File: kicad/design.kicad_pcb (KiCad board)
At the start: 2 copper layers, 20 x 15 mm, 1 part, among them U1 CH32L103K8U6

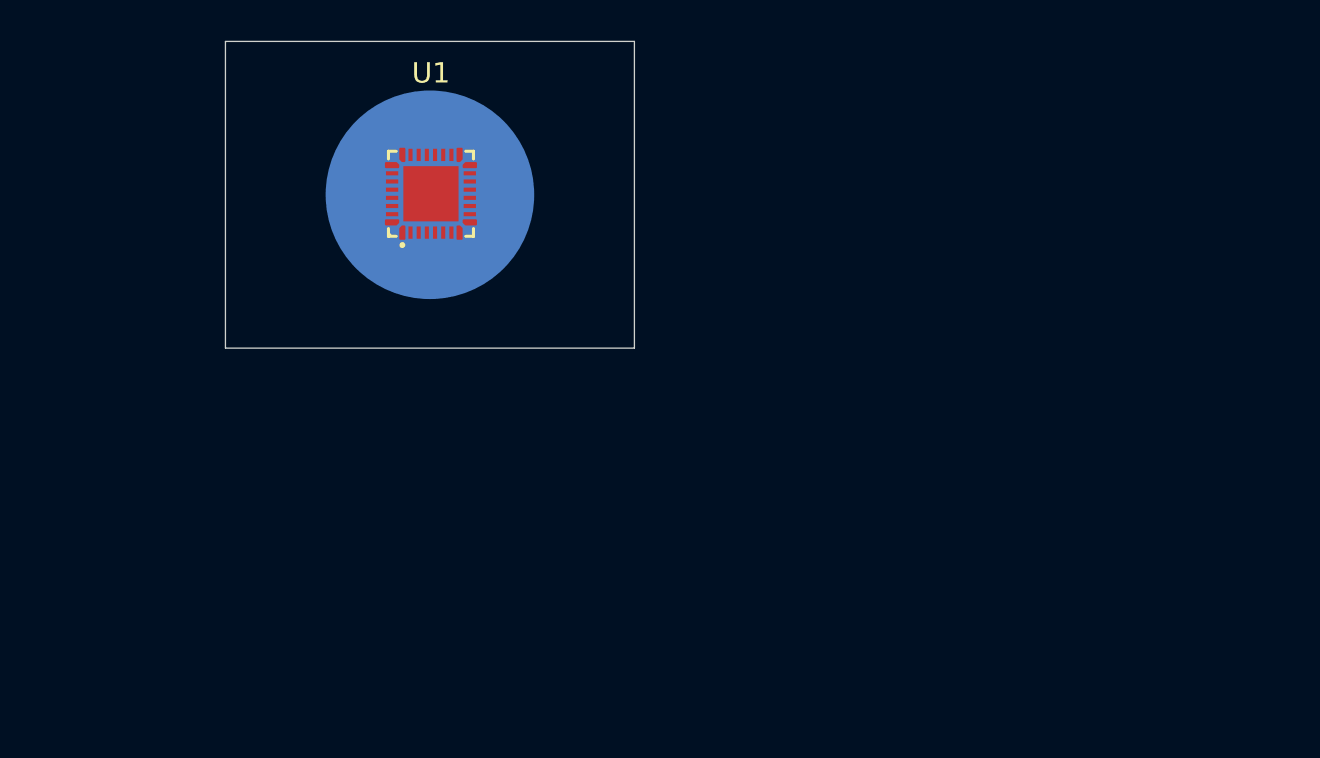
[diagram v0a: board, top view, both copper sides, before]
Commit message: I dont remember last commit idk
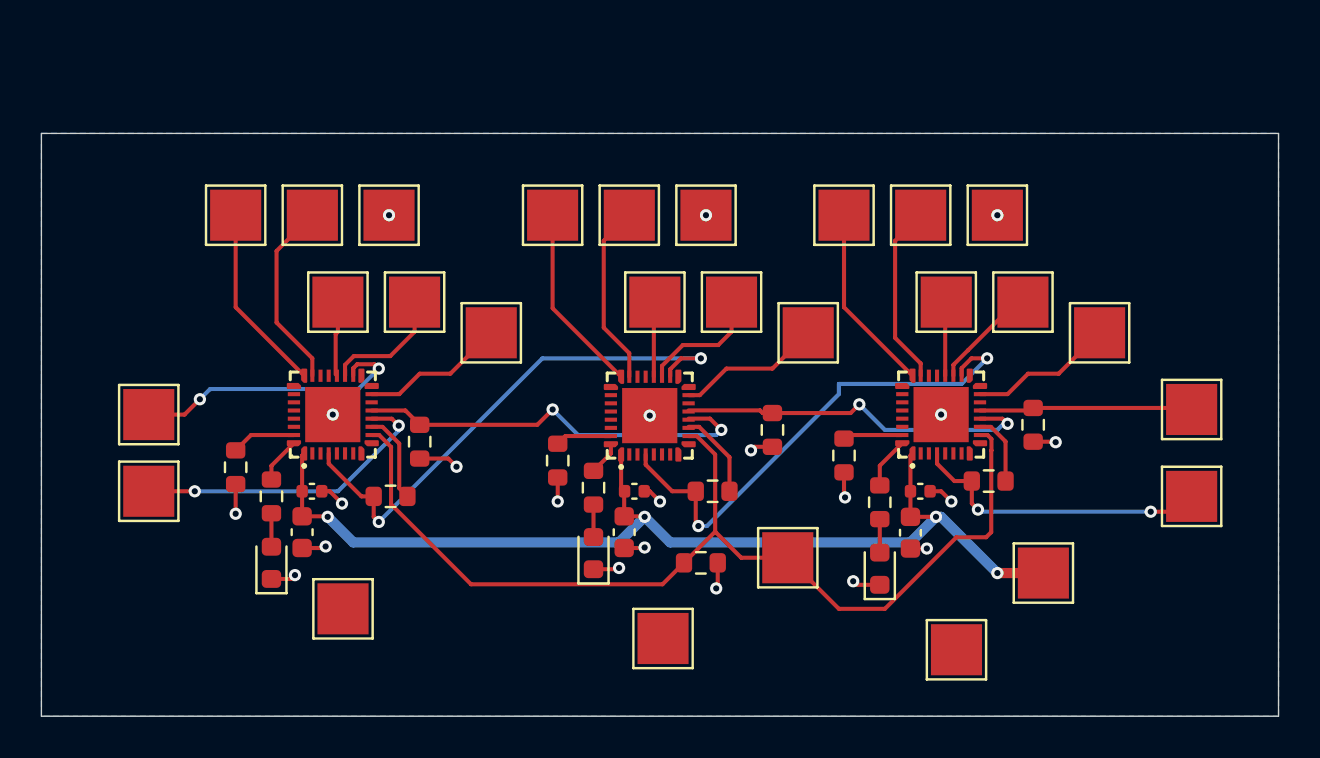
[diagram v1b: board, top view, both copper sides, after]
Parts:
- removed U1: CH32L103K8U6, LIB:QFN-32_L4.0-W4.0-P0.40-BL-EP2.7-A
- added C2: 4.7u, Capacitor_SMD:C_0603_1608Metric, F.Cu at (158.5, 89.0)
- added C3: 0.1u, Capacitor_SMD:C_0402_1005Metric, F.Cu at (159.0, 87.0)
- added C4: 0.1u, Capacitor_SMD:C_0402_1005Metric, F.Cu at (145.0, 87.0)
- added C5: 4.7u, Capacitor_SMD:C_0603_1608Metric, F.Cu at (144.5, 89.0)
- added C6: 0.1u, Capacitor_SMD:C_0402_1005Metric, F.Cu at (129.2, 87.0)
- added C7: 4.7u, Capacitor_SMD:C_0603_1608Metric, F.Cu at (128.8, 89.0)
- added D1: LED, LED_SMD:LED_0603_1608Metric, F.Cu at (157.0, 90.8)
- added D2: LED, LED_SMD:LED_0603_1608Metric, F.Cu at (143.0, 90.0)
- added D3: LED, LED_SMD:LED_0603_1608Metric, F.Cu at (127.2, 90.5)
- added R1: 0, Resistor_SMD:R_0603_1608Metric, F.Cu at (162.3, 86.5)
- added R10: 10k, Resistor_SMD:R_0603_1608Metric, F.Cu at (134.5, 84.6)
- added R11: 470, Resistor_SMD:R_0603_1608Metric, F.Cu at (157.0, 87.5)
- added R12: 470, Resistor_SMD:R_0603_1608Metric, F.Cu at (143.0, 86.8)
- added R13: 470, Resistor_SMD:R_0603_1608Metric, F.Cu at (127.2, 87.2)
- added R2: 4.7k, Resistor_SMD:R_0603_1608Metric, F.Cu at (155.2, 85.2)
- added R3: 4.7k, Resistor_SMD:R_0603_1608Metric, F.Cu at (141.2, 85.5)
- added R4: 4.7k, Resistor_SMD:R_0603_1608Metric, F.Cu at (125.5, 85.8)
- added R5: 10k, Resistor_SMD:R_0603_1608Metric, F.Cu at (148.2, 90.5)
- added R6: 0, Resistor_SMD:R_0603_1608Metric, F.Cu at (148.8, 87.0)
- added R7: 0, Resistor_SMD:R_0603_1608Metric, F.Cu at (133.1, 87.2)
- added R8: 10k, Resistor_SMD:R_0603_1608Metric, F.Cu at (164.5, 83.8)
- added R9: 10k, Resistor_SMD:R_0603_1608Metric, F.Cu at (151.8, 84.0)
- added TP1: TestPoint, TestPoint:TestPoint_Pad_2.5x2.5mm, F.Cu at (121.2, 83.2)
- added TP10: TestPoint, TestPoint:TestPoint_Pad_2.5x2.5mm, F.Cu at (125.5, 73.5)
- added TP11: TestPoint, TestPoint:TestPoint_Pad_2.5x2.5mm, F.Cu at (162.8, 73.5)
- added TP12: TestPoint, TestPoint:TestPoint_Pad_2.5x2.5mm, F.Cu at (148.5, 73.5)
- added TP13: TestPoint, TestPoint:TestPoint_Pad_2.5x2.5mm, F.Cu at (133.0, 73.5)
- added TP14: TestPoint, TestPoint:TestPoint_Pad_2.5x2.5mm, F.Cu at (165.0, 91.0)
- added TP15: TestPoint, TestPoint:TestPoint_Pad_2.5x2.5mm, F.Cu at (152.5, 90.2)
- added TP16: TestPoint, TestPoint:TestPoint_Pad_2.5x2.5mm, F.Cu at (167.8, 79.2)
- added TP17: TestPoint, TestPoint:TestPoint_Pad_2.5x2.5mm, F.Cu at (153.5, 79.2)
- added TP18: TestPoint, TestPoint:TestPoint_Pad_2.5x2.5mm, F.Cu at (138.0, 79.2)
- added TP19: TestPoint, TestPoint:TestPoint_Pad_2.5x2.5mm, F.Cu at (164.0, 77.8)
- added TP2: TestPoint, TestPoint:TestPoint_Pad_2.5x2.5mm, F.Cu at (172.2, 87.2)
- added TP20: TestPoint, TestPoint:TestPoint_Pad_2.5x2.5mm, F.Cu at (149.8, 77.8)
- added TP21: TestPoint, TestPoint:TestPoint_Pad_2.5x2.5mm, F.Cu at (134.2, 77.8)
- added TP22: TestPoint, TestPoint:TestPoint_Pad_2.5x2.5mm, F.Cu at (160.2, 77.8)
- added TP23: TestPoint, TestPoint:TestPoint_Pad_2.5x2.5mm, F.Cu at (146.0, 77.8)
- added TP24: TestPoint, TestPoint:TestPoint_Pad_2.5x2.5mm, F.Cu at (130.5, 77.8)
- added TP25: TestPoint, TestPoint:TestPoint_Pad_2.5x2.5mm, F.Cu at (160.8, 94.8)
- added TP26: TestPoint, TestPoint:TestPoint_Pad_2.5x2.5mm, F.Cu at (146.4, 94.2)
- added TP27: TestPoint, TestPoint:TestPoint_Pad_2.5x2.5mm, F.Cu at (130.8, 92.8)
- added TP3: TestPoint, TestPoint:TestPoint_Pad_2.5x2.5mm, F.Cu at (172.2, 83.0)
- added TP4: TestPoint, TestPoint:TestPoint_Pad_2.5x2.5mm, F.Cu at (121.2, 87.0)
- added TP5: TestPoint, TestPoint:TestPoint_Pad_2.5x2.5mm, F.Cu at (155.2, 73.5)
- added TP6: TestPoint, TestPoint:TestPoint_Pad_2.5x2.5mm, F.Cu at (159.0, 73.5)
- added TP7: TestPoint, TestPoint:TestPoint_Pad_2.5x2.5mm, F.Cu at (144.8, 73.5)
- added TP8: TestPoint, TestPoint:TestPoint_Pad_2.5x2.5mm, F.Cu at (141.0, 73.5)
- added TP9: TestPoint, TestPoint:TestPoint_Pad_2.5x2.5mm, F.Cu at (129.2, 73.5)
- added U2: CH32L103K8U6, LIB:QFN-32_L4.0-W4.0-P0.40-BL-EP2.7-A, F.Cu at (160.0, 83.2)
- added U3: CH32L103K8U6, LIB:QFN-32_L4.0-W4.0-P0.40-BL-EP2.7-A, F.Cu at (145.8, 83.3)
- added U4: CH32L103K8U6, LIB:QFN-32_L4.0-W4.0-P0.40-BL-EP2.7-A, F.Cu at (130.2, 83.2)
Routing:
- net /3v3: track 0.00 -> 51.1 mm, vias 0 -> 4
- net /NSS: track 0.00 -> 49.8 mm
- net /electrode1/CLK_OUT: track 0.00 -> 25.9 mm, vias 0 -> 2
- net /electrode/CLK_OUT: track 0.00 -> 24.9 mm, vias 0 -> 2
- net /electrode1/SPI_MISO: track 0.00 -> 20.2 mm, vias 0 -> 2
- net GND: track 0.00 -> 19.7 mm, vias 0 -> 22
- net /electrode/SPI_MISO: track 0.00 -> 18.2 mm, vias 0 -> 2
- net /electrode2/SPI_MISO: track 0.00 -> 15.2 mm, vias 0 -> 2
- net /electrode/CLK_IN: track 0.00 -> 14.9 mm, vias 0 -> 2
- net /electrode2/CLK_OUT: track 0.00 -> 14.0 mm, vias 0 -> 2
- net /electrode/SPI_MOSI: track 0.00 -> 10.4 mm
- net /electrode2/SWDIO: track 0.00 -> 9.30 mm
- net /electrode1/SWCLK: track 0.00 -> 9.29 mm
- net /electrode2/SWCLK: track 0.00 -> 9.24 mm
- net /electrode/SWCLK: track 0.00 -> 9.24 mm
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- added copper zone on B.Cu, net GND
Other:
- board size 20 x 15 mm -> 60.5 x 28.5 mm
